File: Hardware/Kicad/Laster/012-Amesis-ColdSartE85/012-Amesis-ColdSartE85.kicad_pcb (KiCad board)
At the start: 2 copper layers, 52.1 x 26.5 mm, 12 parts, among them J1 Screw_Terminal_01x02, J2 Conn_01x05_Female, J3 Conn_01x03_Female

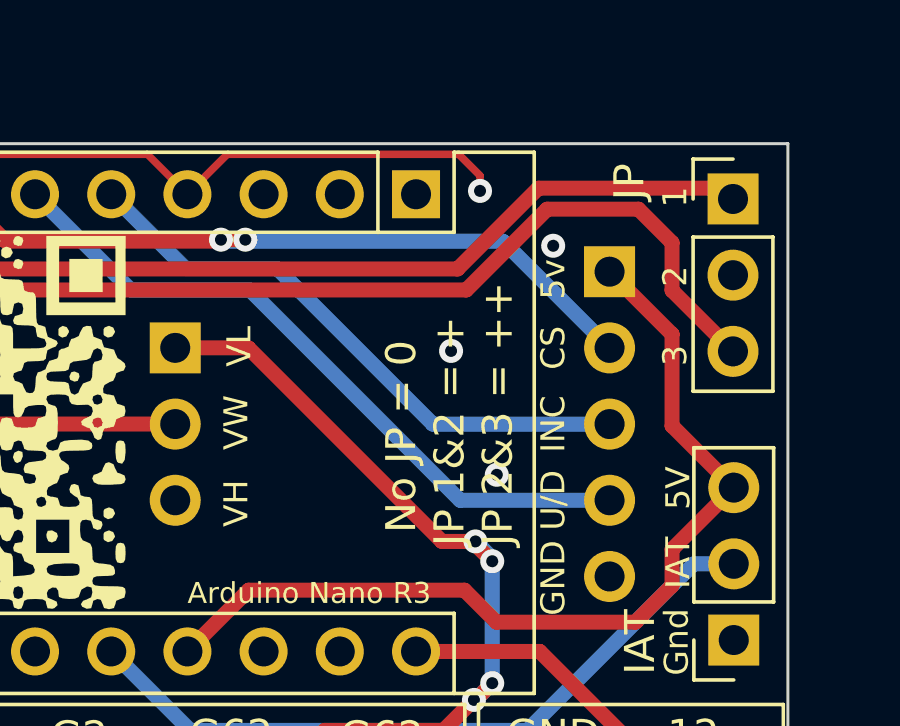
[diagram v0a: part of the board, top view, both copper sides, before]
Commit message: maj pcb et code arduino avec jp et sonde iat
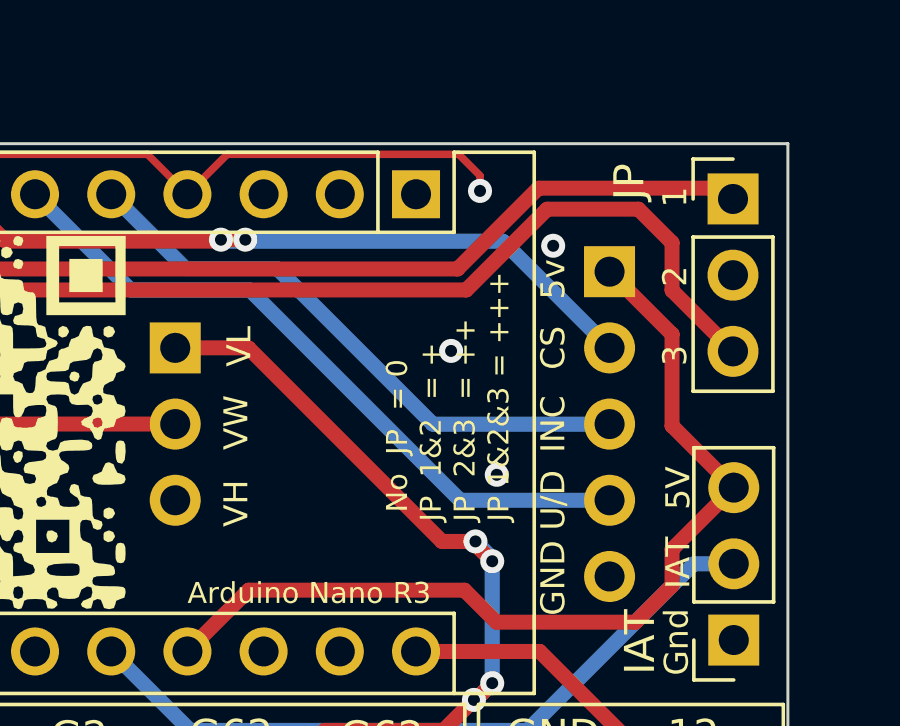
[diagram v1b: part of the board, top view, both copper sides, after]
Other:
- board text added: "No JP = 0 JP 1&2 = + JP 2&3 = ++ JP 1&2&3 = +++"
- board text removed: "No JP = 0 JP 1&2 = + JP 2&3 = ++"
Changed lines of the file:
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@@
       (outputformat 1)
       (mirror false)
-      (drillshape 1)
+      (drillshape 0)
       (scaleselection 1)
-      (outputdirectory "")
+      (outputdirectory "012-Amesis-ColdSartE85-backups/Fichier de prod/")
     )
   )
@@
     (effects (font (size 0.8 0.8) (thickness 0.1)))
   )
-  (gr_text " No JP = 0\nJP 1&2 = +\nJP 2&3 = ++" (at 159.005754 58.370904 90) (layer "F.SilkS")
-    (effects (font (size 1 1) (thickness 0.2)) (justify left))
+  (gr_text " No  JP  = 0\nJP  1&2  = +\nJP  2&3  = ++\nJP 1&2&3 = +++" (at 158.9532 57.5564 90) (layer "F.SilkS")
+    (effects (font (size 0.7 0.7) (thickness 0.175)) (justify left))
+  )
+  (dimension (type aligned) (layer "F.Cu")
+    (pts (xy 170.18 44.959704) (xy 118.213354 44.959704))
+    (height 4.827703)
+    (gr_text "51,9666 mm" (at 144.196677 38.332001) (layer "F.Cu")
+      (effects (font (size 1.5 1.5) (thickness 0.3)))
+    )
+    (format (units 3) (units_format 1) (precision 4))
+    (style (thickness 0.2) (arrow_length 1.27) (text_position_mode 0) (extension_height 0.58642) (extension_offset 0.5) keep_text_aligned)
+  )
+  (dimension (type aligned) (layer "F.Cu")
+    (pts (xy 170.300954 71.464104) (xy 170.283354 44.959704))
+    (height 5.484274)
+    (gr_text "26,5044 mm" (at 177.576427 58.207067 -89.96195328) (layer "F.Cu")
+      (effects (font (size 1.5 1.5) (thickness 0.3)))
+    )
+    (format (units 3) (units_format 1) (precision 4))
+    (style (thickness 0.2) (arrow_length 1.27) (text_position_mode 0) (extension_height 0.58642) (extension_offset 0.5) keep_text_aligned)
   )
   (segment (start 151.598954 45.315304) (end 150.268154 46.646104) (width 0.25) (layer "F.Cu") (net 7))

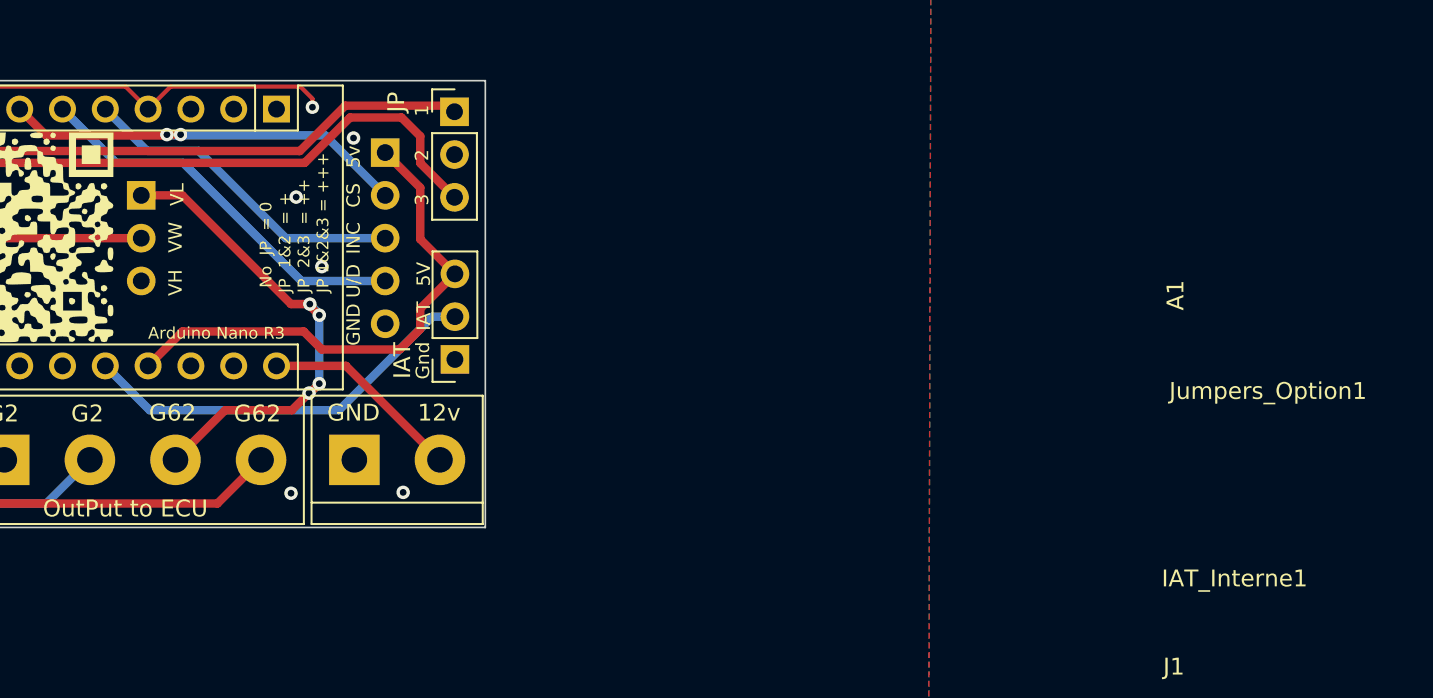
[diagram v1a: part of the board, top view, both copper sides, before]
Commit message: code v0.02
termista
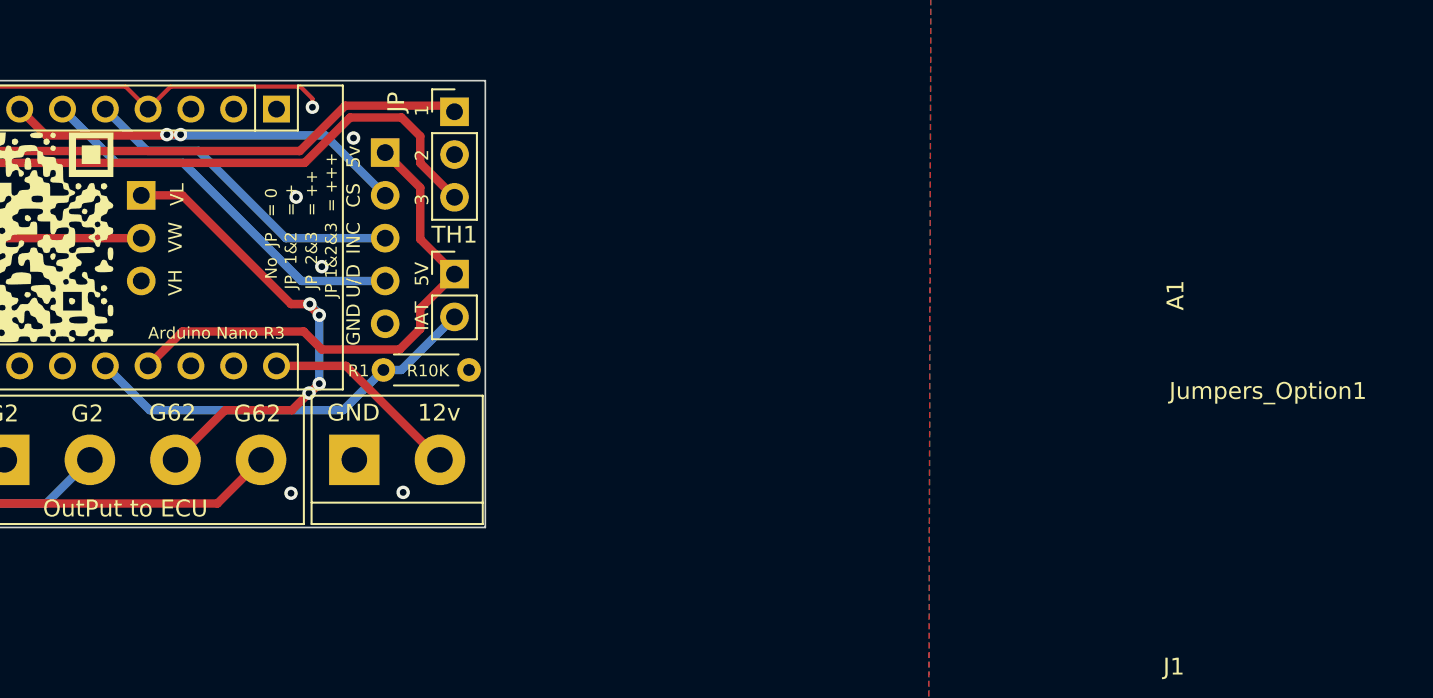
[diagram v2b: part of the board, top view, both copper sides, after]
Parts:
- removed IAT_Interne1: R_Potentiometer, Connector_PinSocket_2.54mm:PinSocket_1x03_P2.54mm_Vertical
- added R1: R10K, Resistor_THT:R_Axial_DIN0204_L3.6mm_D1.6mm_P5.08mm_Horizontal, F.Cu at (164.2, 62.1)
- added TH1: Thermistor, Connector_PinHeader_2.54mm:PinHeader_1x02_P2.54mm_Vertical, F.Cu at (168.5, 56.4)
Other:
- board text added: "JP 1&2 = +"
- board text added: "JP 1&2&3 = +++"
- board text added: "JP 2&3 = ++"
- board text added: "No JP = 0"
- board text removed: "No JP = 0 JP 1&2 = + JP 2&3 = ++ JP 1&2&3 = +++"
